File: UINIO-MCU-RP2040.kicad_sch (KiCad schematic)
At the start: 46 parts, among them J1 Conn_01x20_Pin, J2 Conn_01x20_Pin, J3 Conn_01x04_Pin, Q1 DMG1012T, SW1 ~{RESET}, SW2 ~{USB_BOOT}, U1 SGM2019-3.3YN5G, U2 SPI-25-Flash-WSON8, U3 RP2040, Y1 12MHz

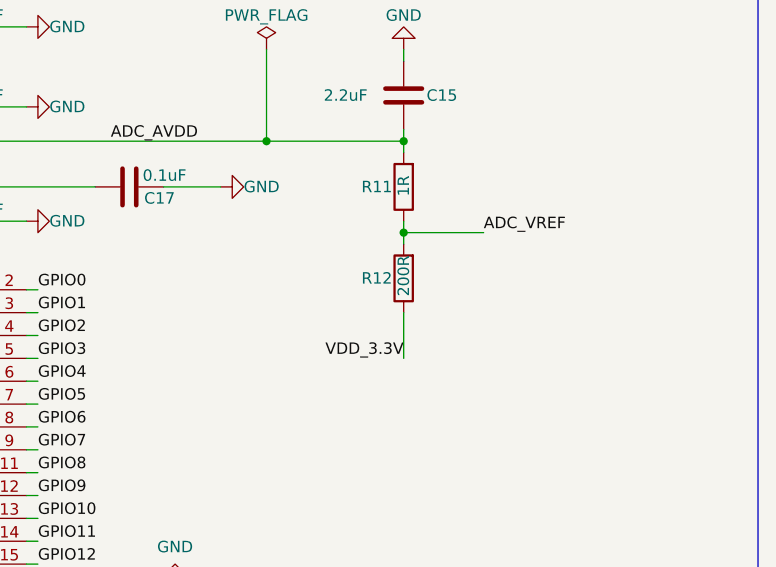
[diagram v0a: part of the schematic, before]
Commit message: Release UINIO-MCU-RP2040 version 3.2.0.
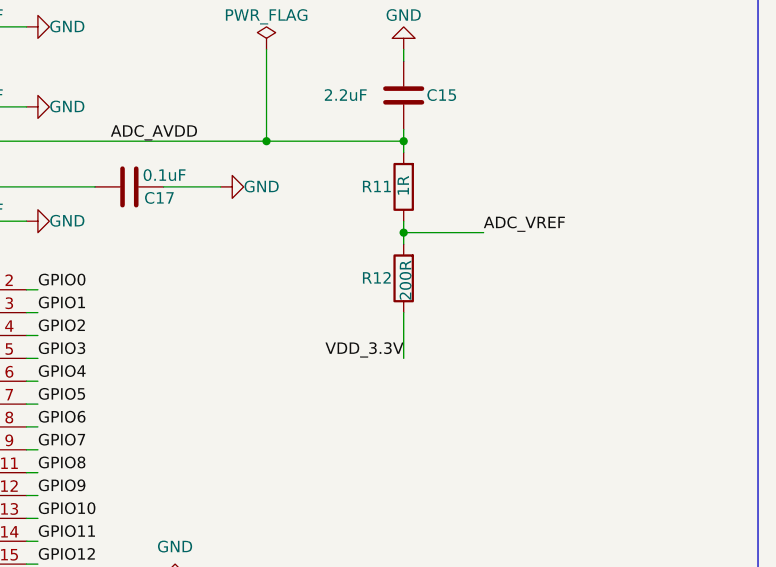
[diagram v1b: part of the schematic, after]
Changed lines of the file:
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@@
 		)
 		(property "Value" "200R"
-			(at 358.14 76.2 90)
+			(at 358.394 76.708 90)
 			(effects
 				(font
